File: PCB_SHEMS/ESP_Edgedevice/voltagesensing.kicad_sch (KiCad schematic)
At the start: 36 parts, among them J4 Conn_01x02, U3 AMS1117-5.0, U4 AMC1200SDUBR, U5 OPA333xxDBV, U6 OPA333xxDBV, U7 MCP3202

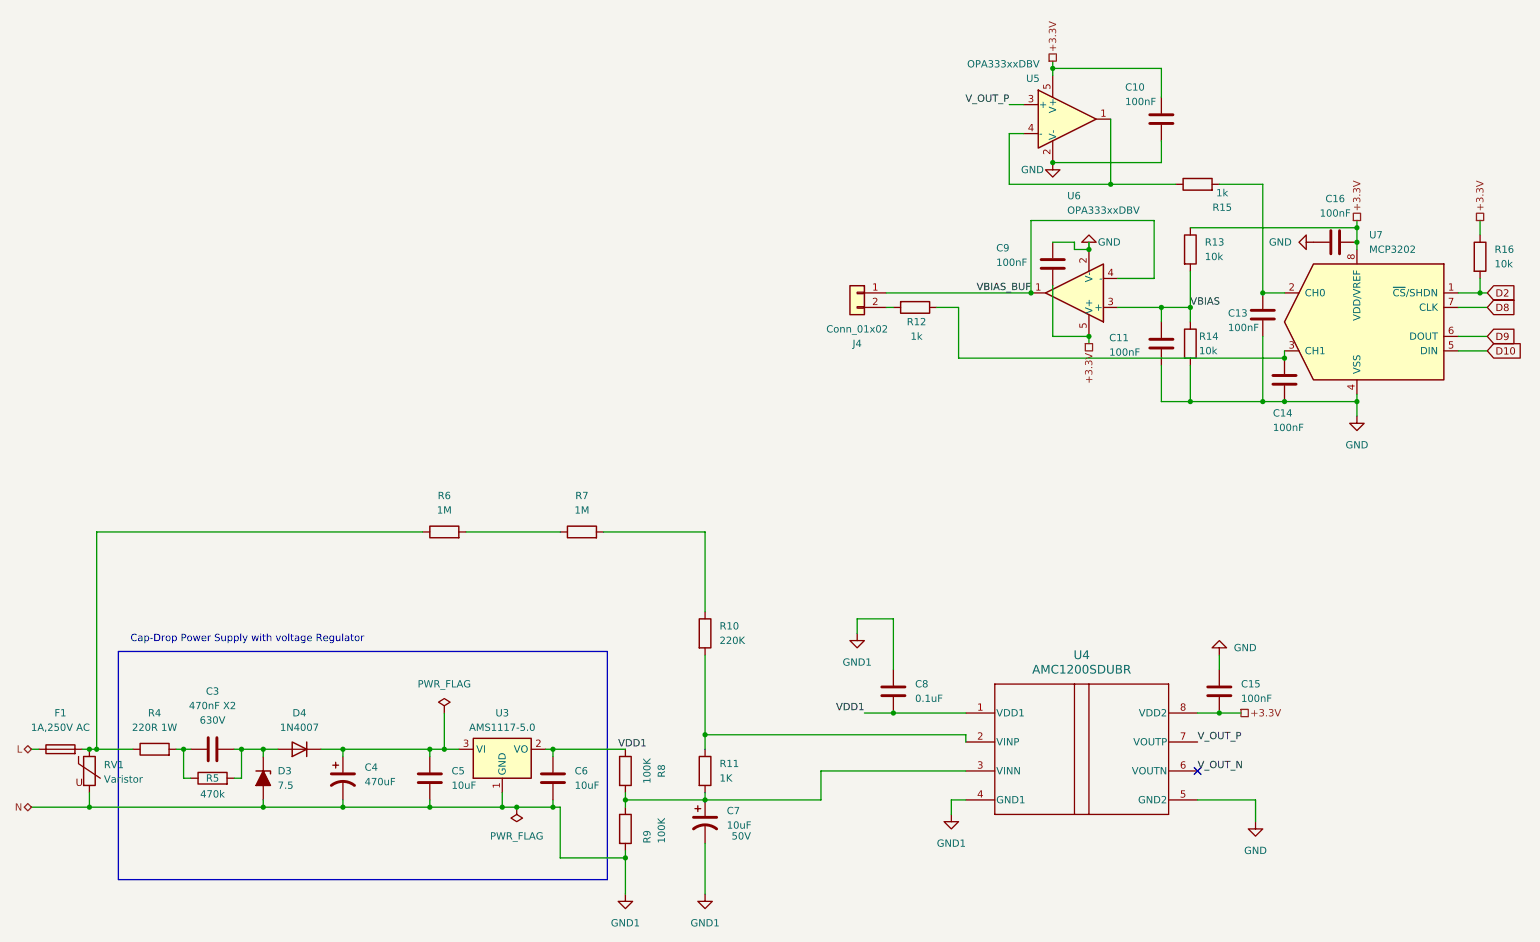
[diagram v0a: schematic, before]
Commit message: made more Schema changes in Lab
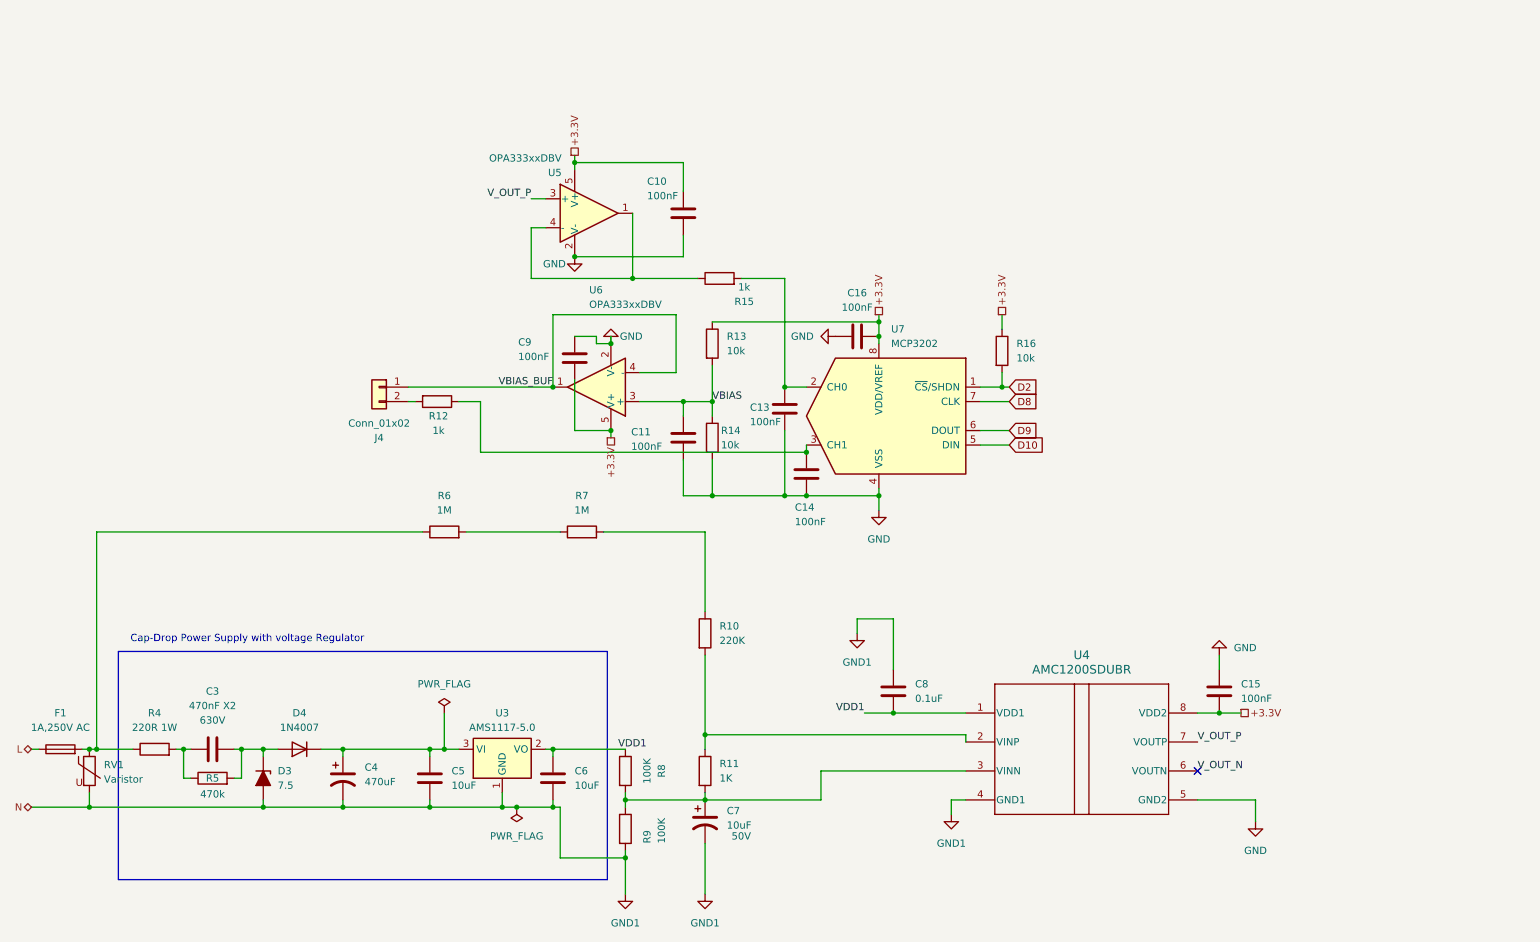
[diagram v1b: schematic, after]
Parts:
- C10, C11, C13, C14, C15, C8: footprint Capacitor_THT:C_Disc_D5.0mm_W2.5mm_P5.00mm -> Capacitor_SMD:C_1206_3216Metric
- C16, C9: footprint Capacitor_SMD:C_0805_2012Metric -> Capacitor_SMD:C_1206_3216Metric
- C5: footprint Capacitor_THT:CP_Radial_D10.0mm_P5.00mm -> Capacitor_SMD:C_1206_3216Metric
- C6: footprint Capacitor_THT:C_Disc_D5.0mm_W2.5mm_P5.00mm -> Capacitor_THT:CP_Radial_D5.0mm_P2.50mm
- R10, R11, R12, R13, R14, R15, R16, R8, R9: footprint Resistor_THT:R_Axial_DIN0207_L6.3mm_D2.5mm_P10.16mm_Horizontal -> Resistor_SMD:R_1206_3216Metric
- U7: footprint Package_SO:TSSOP-8_3x3mm_P0.65mm -> Package_SO:TSSOP-8_4.4x3mm_P0.65mm
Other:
- moved on the sheet: C10, C11, C13, C14, C16, C9, J4, R12, R13, R14, R15, R16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
